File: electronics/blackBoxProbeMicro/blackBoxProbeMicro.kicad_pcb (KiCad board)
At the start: 4 copper layers, 29 x 29 mm, 60 parts, among them J1 USB-C, J2 JTAG_2X05, J3 JTAG_2X05, J4 DevBoardUartOutput, Q1 Q_NMOS_DUAL, Q2 Q_PMOS_DUAL, U1 MCP1702-MB, U2 USBLC6-2, U3 STM32F103CBT, Y1 8MHz

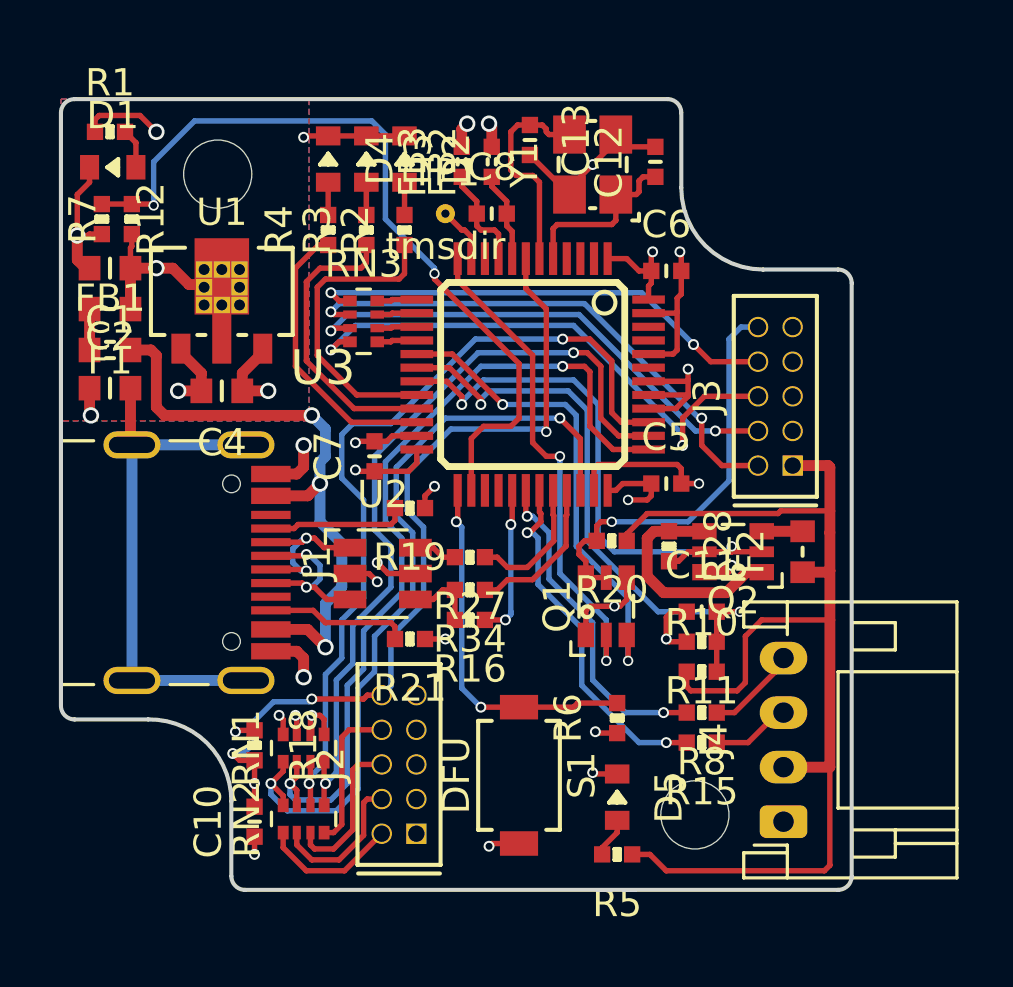
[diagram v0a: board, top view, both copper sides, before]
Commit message: silk optimizations
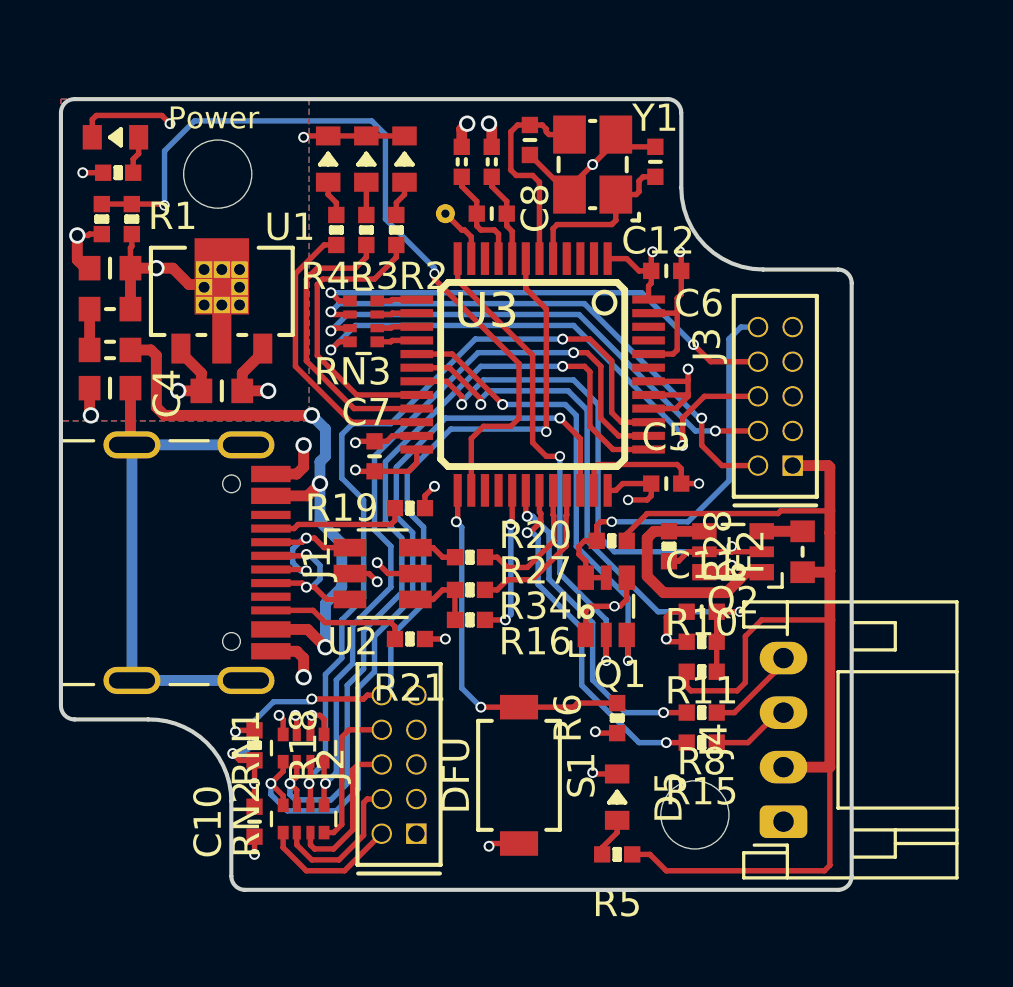
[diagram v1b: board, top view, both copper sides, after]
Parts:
- moved R1 1.53 mm to (135.1, 89.7)
- moved D1 1.10 mm to (135.0, 88.4)
- moved R2 0.30 mm to (145.3, 91.8)
- moved R4 0.30 mm to (143.1, 91.8)
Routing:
- net /VDD: track 27.1 -> 24.8 mm
- net /VSS: track 49.7 -> 50.7 mm, vias 20 -> 21
- net /LED0: track 11.2 -> 10.6 mm
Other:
- board text added: "Power"
